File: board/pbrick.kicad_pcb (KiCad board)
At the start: 4 copper layers, 24 x 44 mm, 58 parts, among them J1 UJC-HP-3-SMT-TR, J2 TC2030-IDC-NL, J3 U.FL2PIN, J4 QWIIC, J5 5055670271, M0 5055680471, M1 5055680471, Q1 SSM6J507NU, Q2 SSM6J507NU, U1 MIC5219-3.3YML-TR, U2 ADP3330ARTZ-5-RL7, U3 STUSB4500QTR, U5 TB67H420FTG(O,EL), U6 2533020201601, U7 PCA9624, U8 ESDA25W5

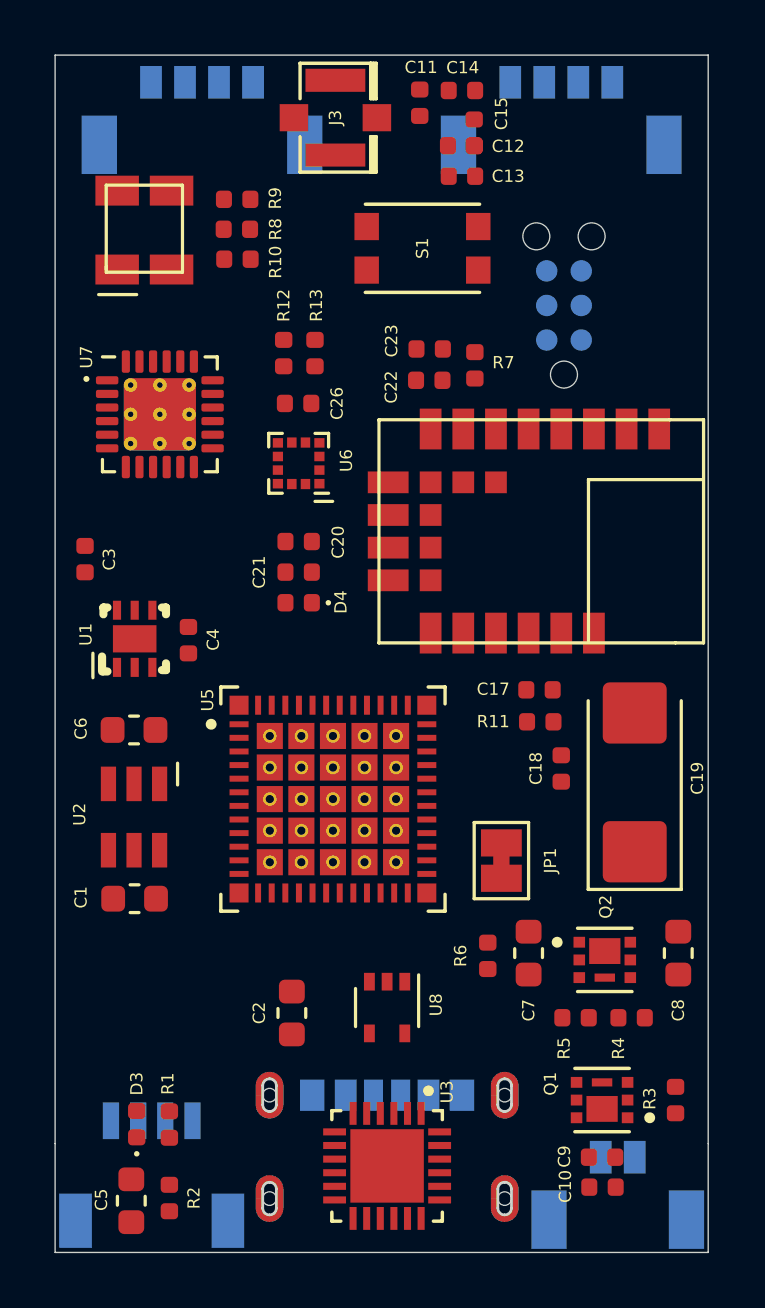
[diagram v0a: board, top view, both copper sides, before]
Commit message: New routing
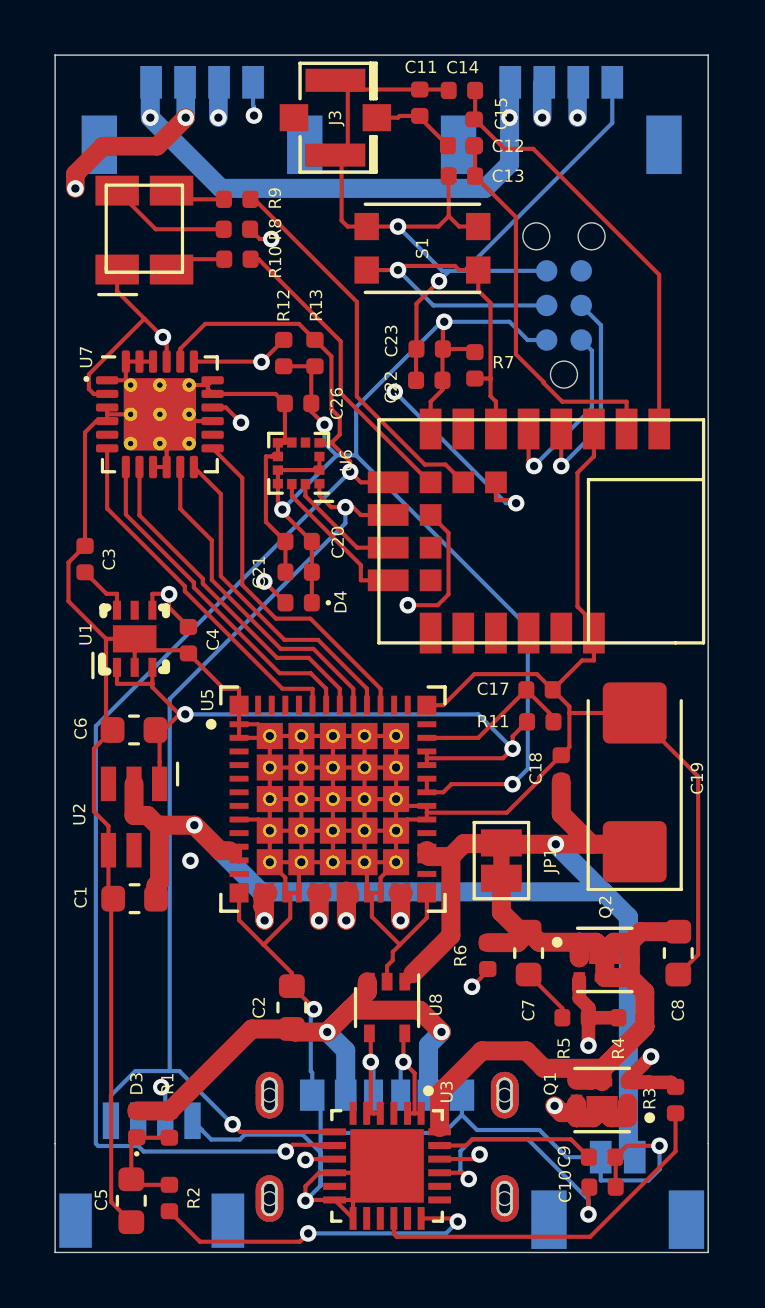
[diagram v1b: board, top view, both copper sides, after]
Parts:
- moved C2 0.20 mm to (128.7, 125.0)
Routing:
- net GND: track 0.00 -> 277.9 mm, vias 0 -> 6
- net VDD: track 0.00 -> 115.4 mm, vias 0 -> 4
- net 3.3V: track 0.00 -> 84.9 mm, vias 0 -> 6
- net /P0.19: track 0.00 -> 52.2 mm, vias 0 -> 2
- net 5V: track 0.00 -> 47.4 mm, vias 0 -> 3
- net /P0.22: track 0.00 -> 47.4 mm, vias 0 -> 3
- net /M0_0: track 0.00 -> 40.3 mm, vias 0 -> 2
- net /M1_1: track 0.00 -> 39.3 mm, vias 0 -> 4
- net /M1_0: track 0.00 -> 37.7 mm, vias 0 -> 2
- net /M0_1: track 0.00 -> 36.2 mm, vias 0 -> 2
- net VSS: track 0.00 -> 33.1 mm
- net VBUS: track 0.00 -> 31.4 mm, vias 0 -> 3
- net /P0.18: track 0.00 -> 16.9 mm, vias 0 -> 1
- net /P0.09: track 0.00 -> 16.0 mm, vias 0 -> 3
- net /ANT: track 0.00 -> 15.9 mm
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- removed copper zone on M.Cu, net VBUS
